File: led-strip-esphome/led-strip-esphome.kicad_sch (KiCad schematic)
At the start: 26 parts, among them Q1 FS8205A_C2830320, U1 TP4056_C725790, U2 BL8072COTR33, U3 AI-WB2-12F, U5 DW01A

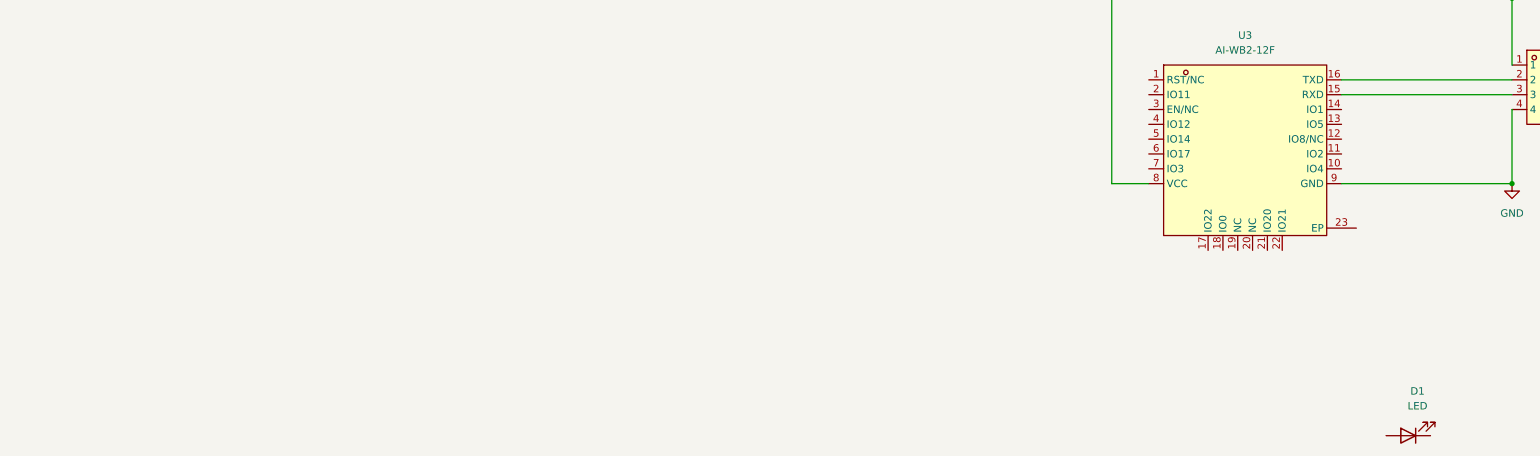
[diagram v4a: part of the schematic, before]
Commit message: pcb
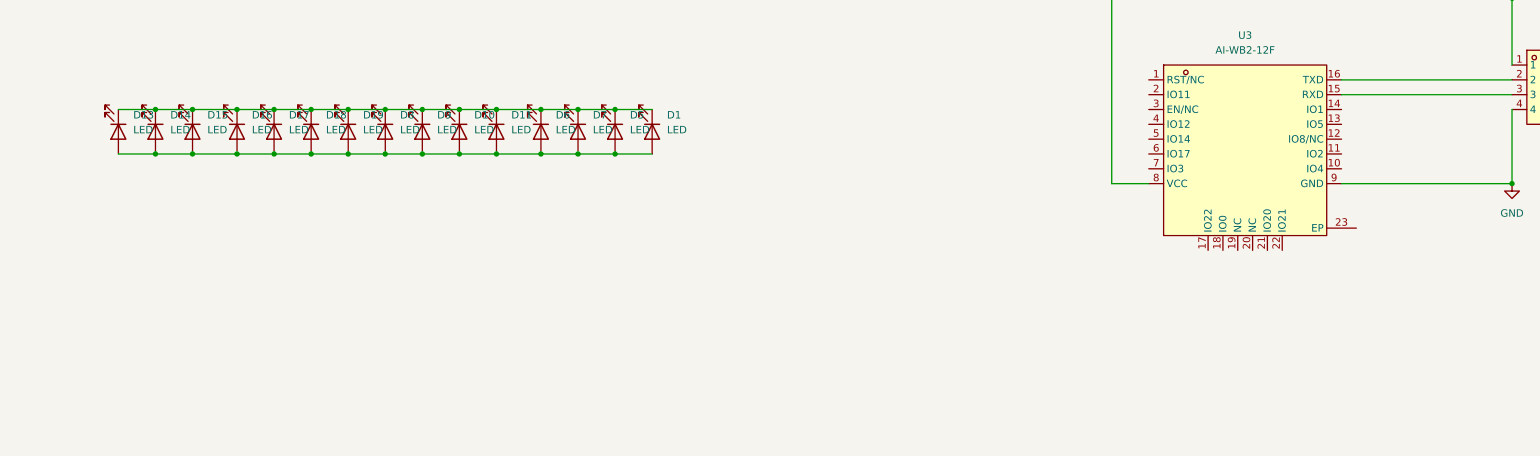
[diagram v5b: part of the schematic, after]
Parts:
- added D10, D11, D13, D14, D15, D16, D17, D18, D19, D5, D6, D7, D8, D9: LED, LED_SMD:LED_PLCC_2835, symbol Device:LED
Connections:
- net at D1.1 (K): now also D10.1 (K), D11.1 (K), D13.1 (K), D14.1 (K), D15.1 (K), D16.1 (K), D17.1 (K), D18.1 (K), D19.1 (K), D5.1 (K), D6.1 (K), D7.1 (K), D8.1 (K), D9.1 (K)
- net at D1.2 (A): now also D10.2 (A), D11.2 (A), D13.2 (A), D14.2 (A), D15.2 (A), D16.2 (A), D17.2 (A), D18.2 (A), D19.2 (A), D5.2 (A), D6.2 (A), D7.2 (A), D8.2 (A), D9.2 (A)
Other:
- moved on the sheet: D1

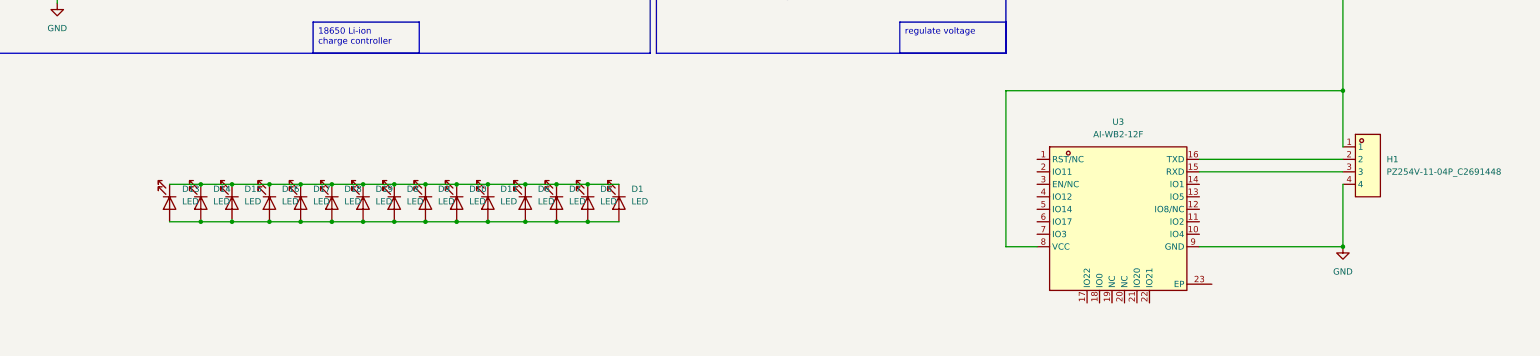
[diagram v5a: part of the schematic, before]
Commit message: schematic finished
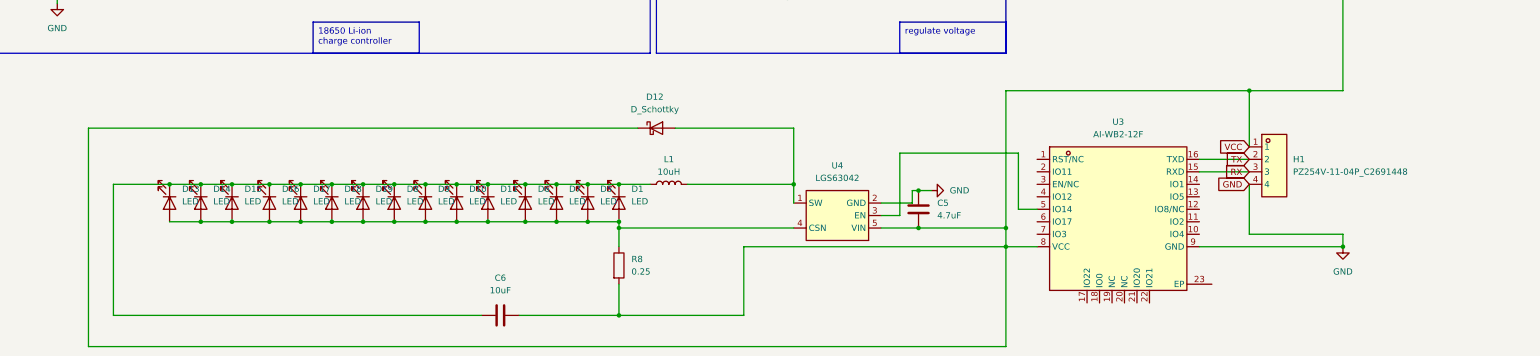
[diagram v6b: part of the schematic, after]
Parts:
- added C5: 4.7uF, symbol Device:C
- added C6: 10uF, symbol Device:C
- added D12: D_Schottky, symbol Device:D_Schottky
- added L1: 10uH, symbol Device:L
- added R8: 0.25, symbol Device:R
- added U4: LGS63042, easyeda2kicad:SOT-23-5_L2.9-W1.6-P0.95-LS2.8-BL, symbol easyeda2kicad:LGS63042
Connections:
- net +3.3V: now also C5.2, C6.2, D12.1 (K), R8.2, U4.5 (VIN)
- net GND: now also C5.1, U4.2 (GND)
- net RX: now reaches H1.3, U3.15 (RXD)
- net TX: now reaches H1.2, U3.16 (TXD)
- net at U3.5 (IO14): now also U4.3 (EN)
- net at D1.1 (K), D10.1 (K), D11.1 (K)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: now also C6.1, L1.1
- net at D1.2 (A), D10.2 (A), D11.2 (A)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: now also R8.1, U4.4 (CSN)
- new net: D12.2 (A), L1.2, U4.1 (SW)
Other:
- moved on the sheet: H1

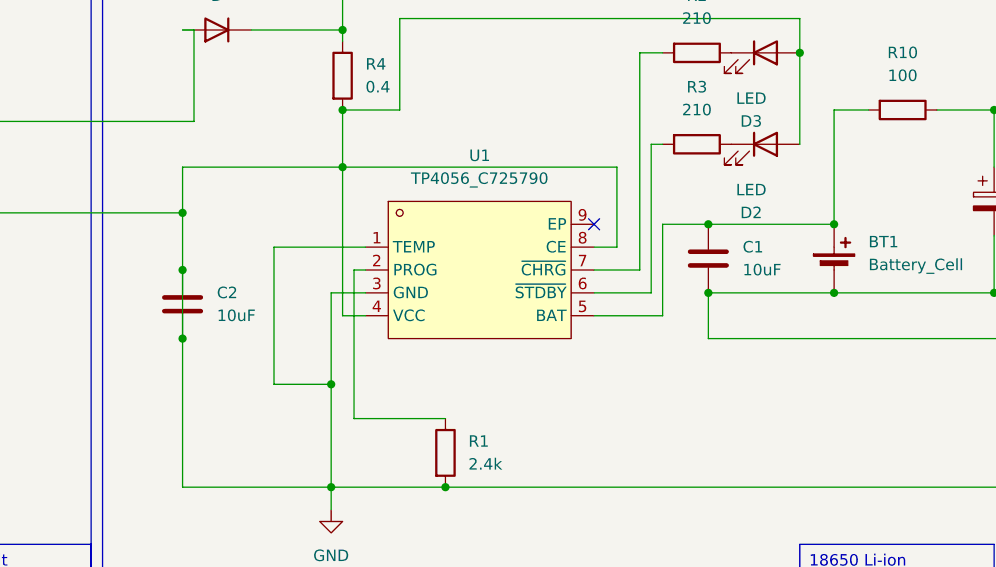
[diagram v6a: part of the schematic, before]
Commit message: add footprints
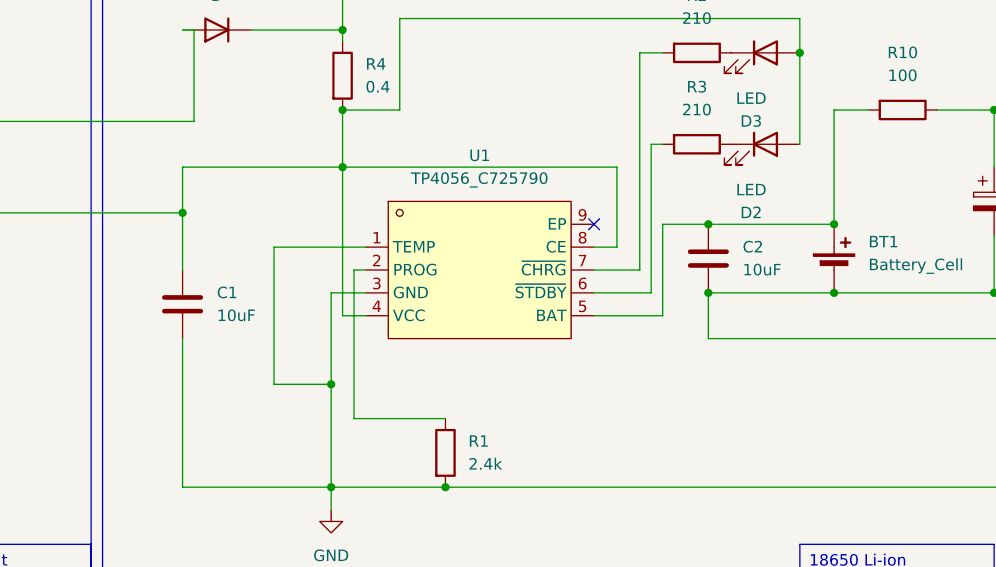
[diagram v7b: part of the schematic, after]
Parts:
- C1, C2, C6: footprint (none) -> Capacitor_SMD:C_0805_2012Metric
- D12: footprint (none) -> Diode_SMD:D_SMA; LCSC (none) -> C5350986
- L1: footprint (none) -> Inductor_SMD:L_Ferrocore_DLG-0403; LCSC (none) -> C2929419
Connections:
- net GND: now also C1.1; no longer C2.1, C2.2, D2.2 (A), D3.2 (A), R4.2, U1.4 (VCC), U1.8 (CE), USB1.A12 (GND), USB1.B12 (GND)
- net at BT1.1 (+), R10.2, U1.5 (BAT): now also C2.2; no longer C1.1
- net at BT1.2 (-), C9.2, Q1.1 (S1)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: now also C2.1; no longer C1.2
- new net: C1.2, D2.2 (A), D3.2 (A), R4.2, U1.4 (VCC), U1.8 (CE), USB1.A12 (GND), USB1.B12 (GND)
